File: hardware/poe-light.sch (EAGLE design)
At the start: 44 parts, among them J1 RJ45-8-SHIELD-PTH, U1 TPS2378

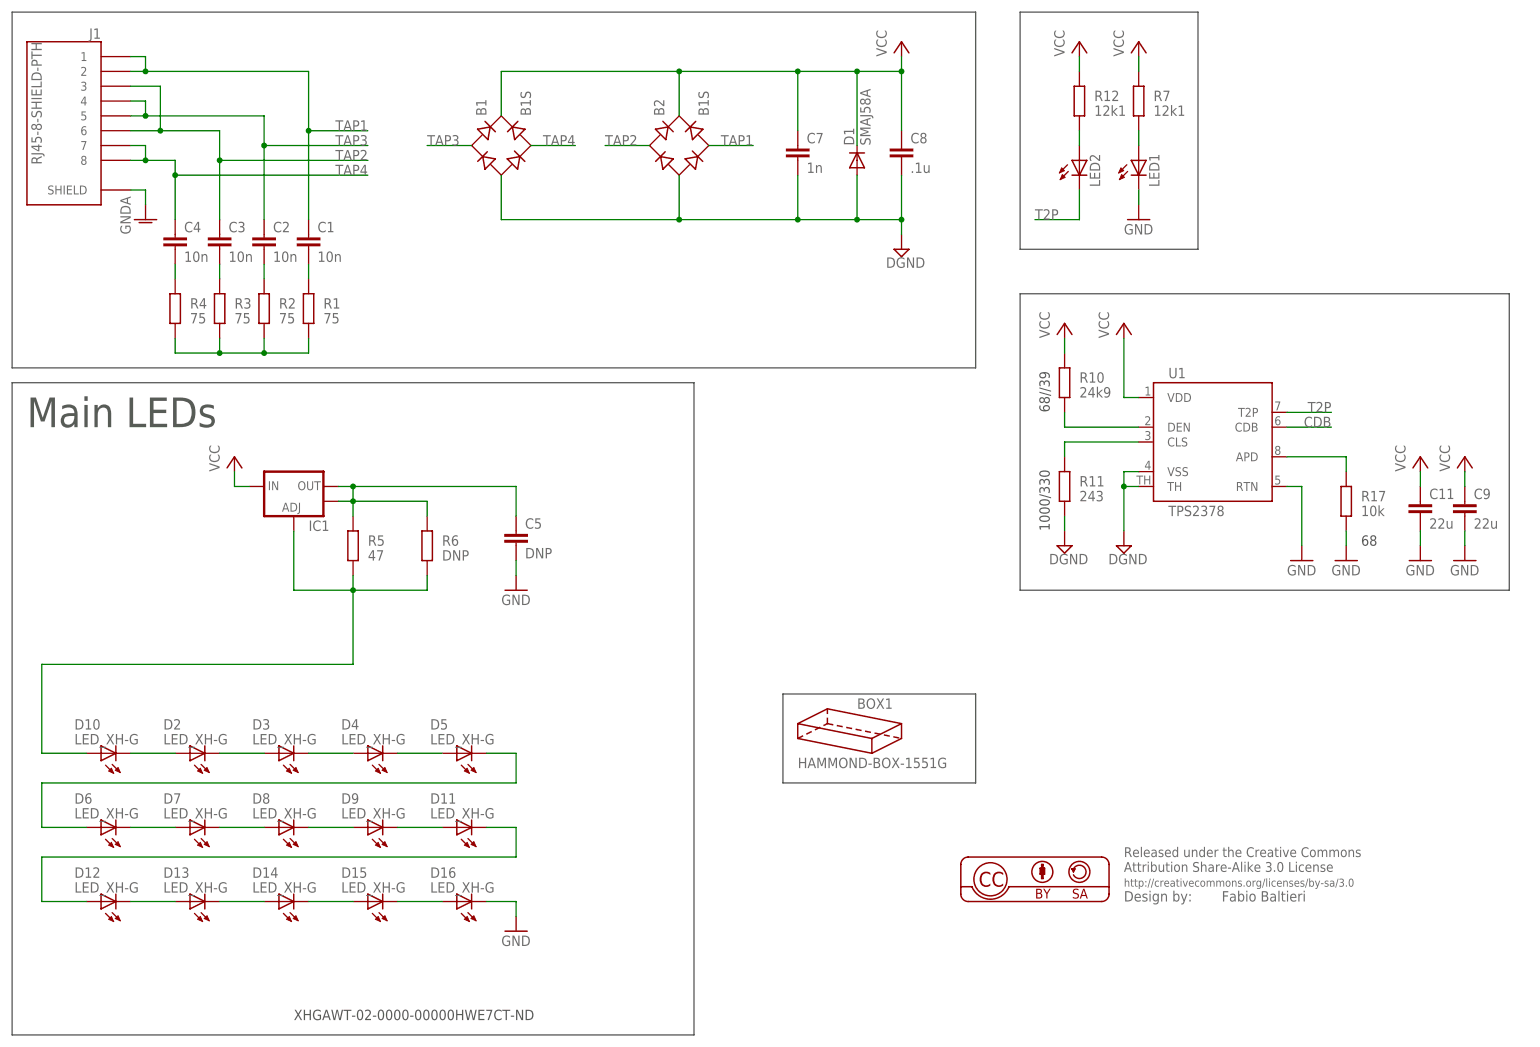
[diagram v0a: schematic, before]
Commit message: hw: sch: layout clean
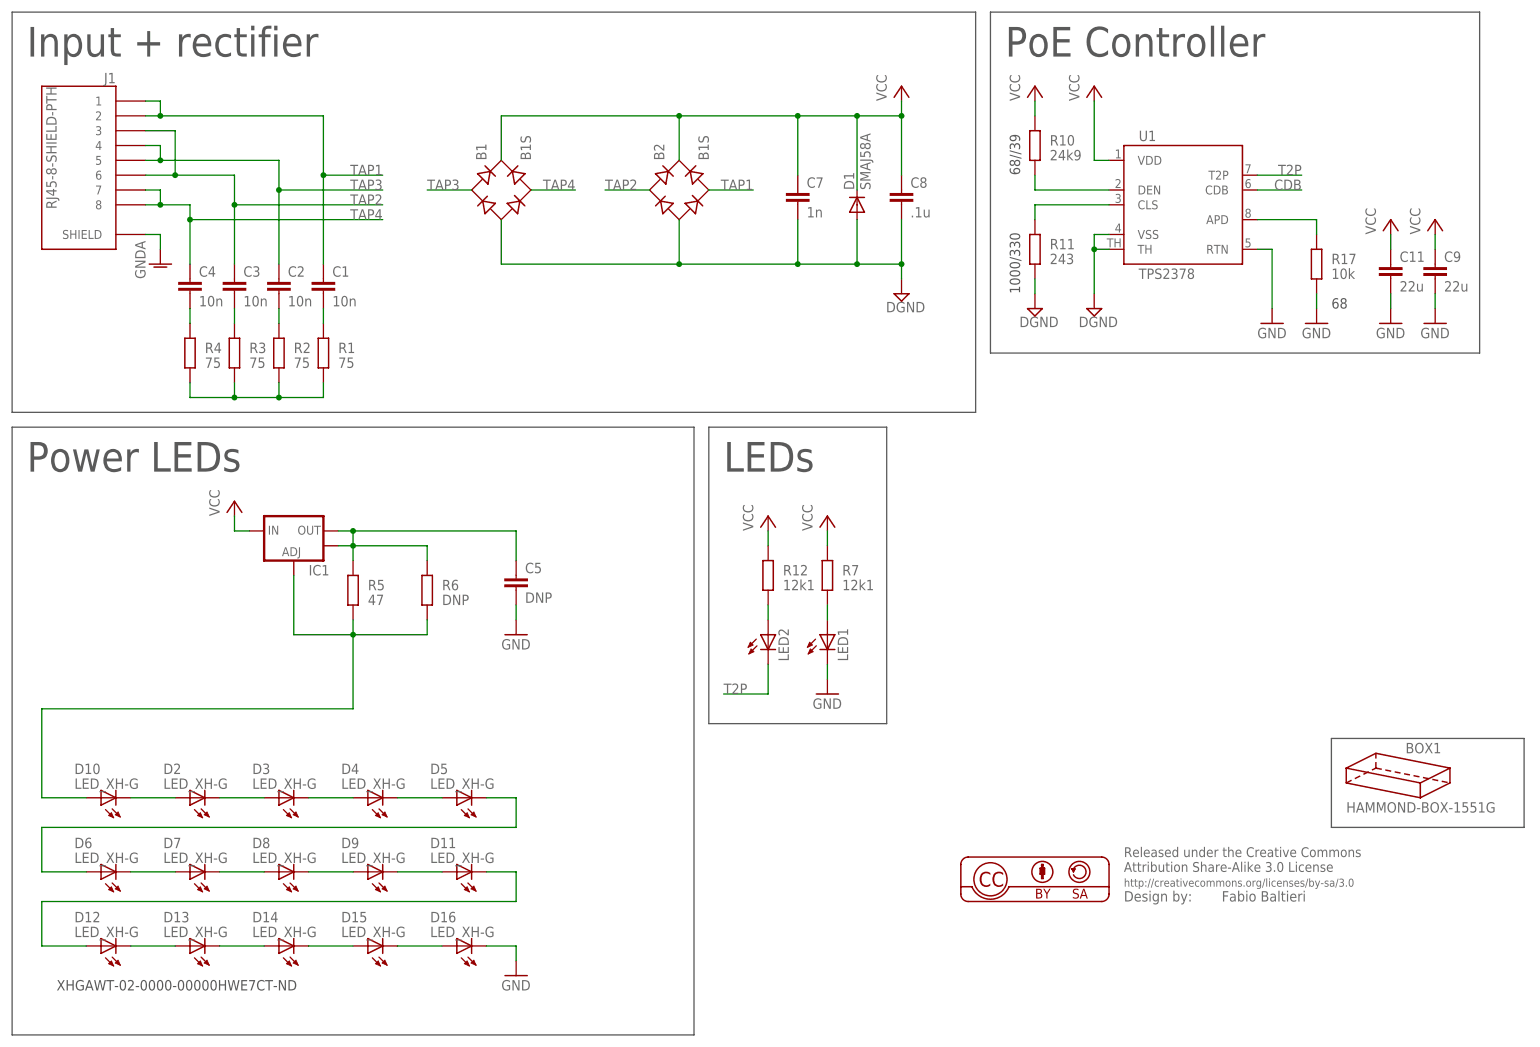
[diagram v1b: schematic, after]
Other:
- note added: "Input + rectifier"
- note added: "LEDs"
- note added: "PoE Controller"
- note added: "Power LEDs"
- note removed: "Main LEDs"
- moved on the sheet: B1, B2, BOX1, C1, C11, C2, C3, C4, C5, C7, C8, C9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
